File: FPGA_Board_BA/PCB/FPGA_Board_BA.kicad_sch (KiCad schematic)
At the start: 3 parts

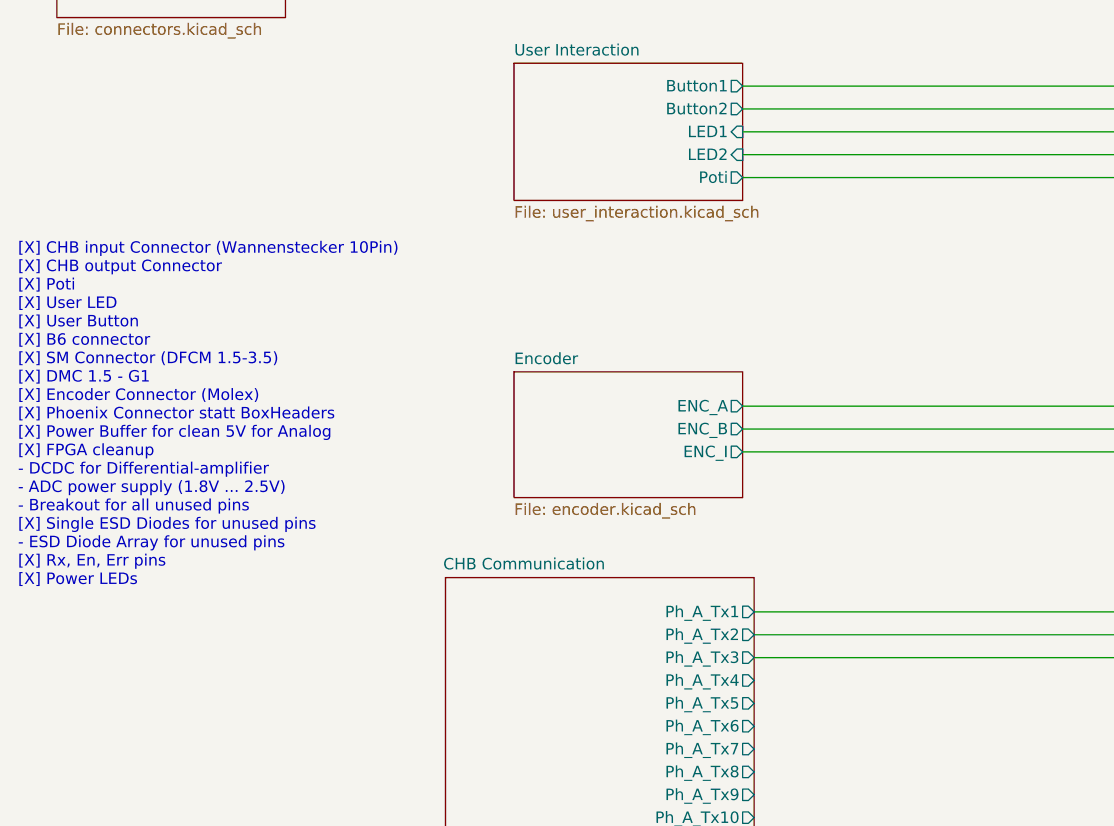
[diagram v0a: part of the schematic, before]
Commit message: Besprechung mit Leo
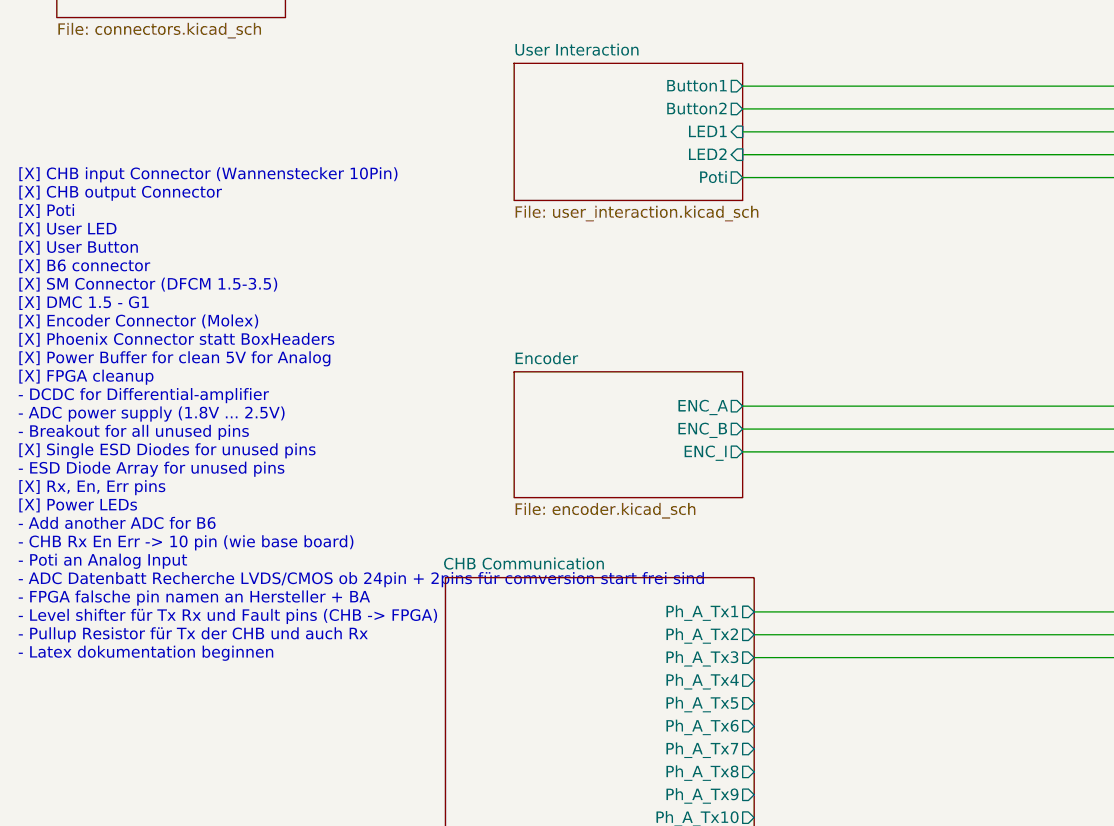
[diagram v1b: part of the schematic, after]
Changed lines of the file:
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@@
 	(generator_version "9.0")
 	(paper "A3")
-	(text "[X] CHB input Connector (Wannenstecker 10Pin)\n[X] CHB output Connector\n[X] Poti\n[X] User LED\n[X] User Button\n[X] B6 connector\n[X] SM Connector (DFCM 1.5-3.5)\n[X] DMC 1.5 - G1\n[X] Encoder Connector (Molex)\n[X] Phoenix Connector statt BoxHeaders\n[X] Power Buffer for clean 5V for Analog\n[X] FPGA cleanup\n- DCDC for Differential-amplifier\n- ADC power supply (1.8V ... 2.5V)\n- Breakout for all unused pins\n[X] Single ESD Diodes for unused pins\n- ESD Diode Array for unused pins\n[X] Rx, En, Err pins\n[X] Power LEDs"
+	(text "[X] CHB input Connector (Wannenstecker 10Pin)\n[X] CHB output Connector\n[X] Poti\n[X] User LED\n[X] User Button\n[X] B6 connector\n[X] SM Connector (DFCM 1.5-3.5)\n[X] DMC 1.5 - G1\n[X] Encoder Connector (Molex)\n[X] Phoenix Connector statt BoxHeaders\n[X] Power Buffer for clean 5V for Analog\n[X] FPGA cleanup\n- DCDC for Differential-amplifier\n- ADC power supply (1.8V ... 2.5V)\n- Breakout for all unused pins\n[X] Single ESD Diodes for unused pins\n- ESD Diode Array for unused pins\n[X] Rx, En, Err pins\n[X] Power LEDs\n- Add another ADC for B6\n- CHB Rx En Err -> 10 pin (wie base board)\n- Poti an Analog Input\n- ADC Datenbatt Recherche LVDS/CMOS ob 24pin + 2pins für comversion start frei sind\n- FPGA falsche pin namen an Hersteller + BA \n- Level shifter für Tx Rx und Fault pins (CHB -> FPGA)\n- Pullup Resistor für Tx der CHB und auch Rx\n- Latex dokumentation beginnen"
 		(exclude_from_sim no)
 		(at 28.702 98.806 0)
